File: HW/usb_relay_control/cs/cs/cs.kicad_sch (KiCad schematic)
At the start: 116 parts

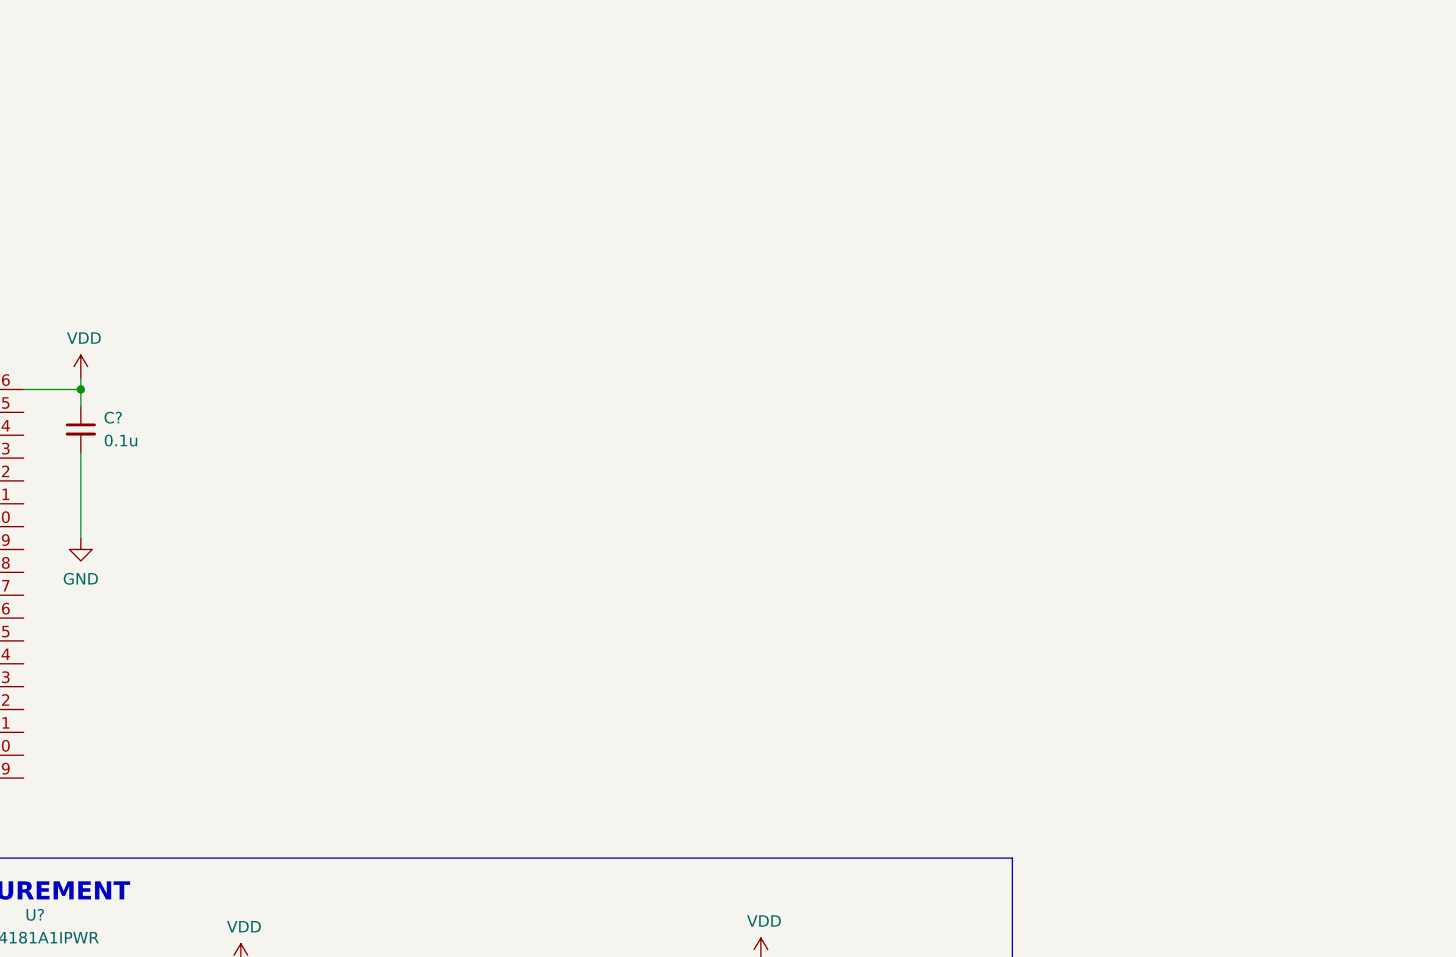
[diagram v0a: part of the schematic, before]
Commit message: ADD: AI antigravity review EMC according to IPC2221
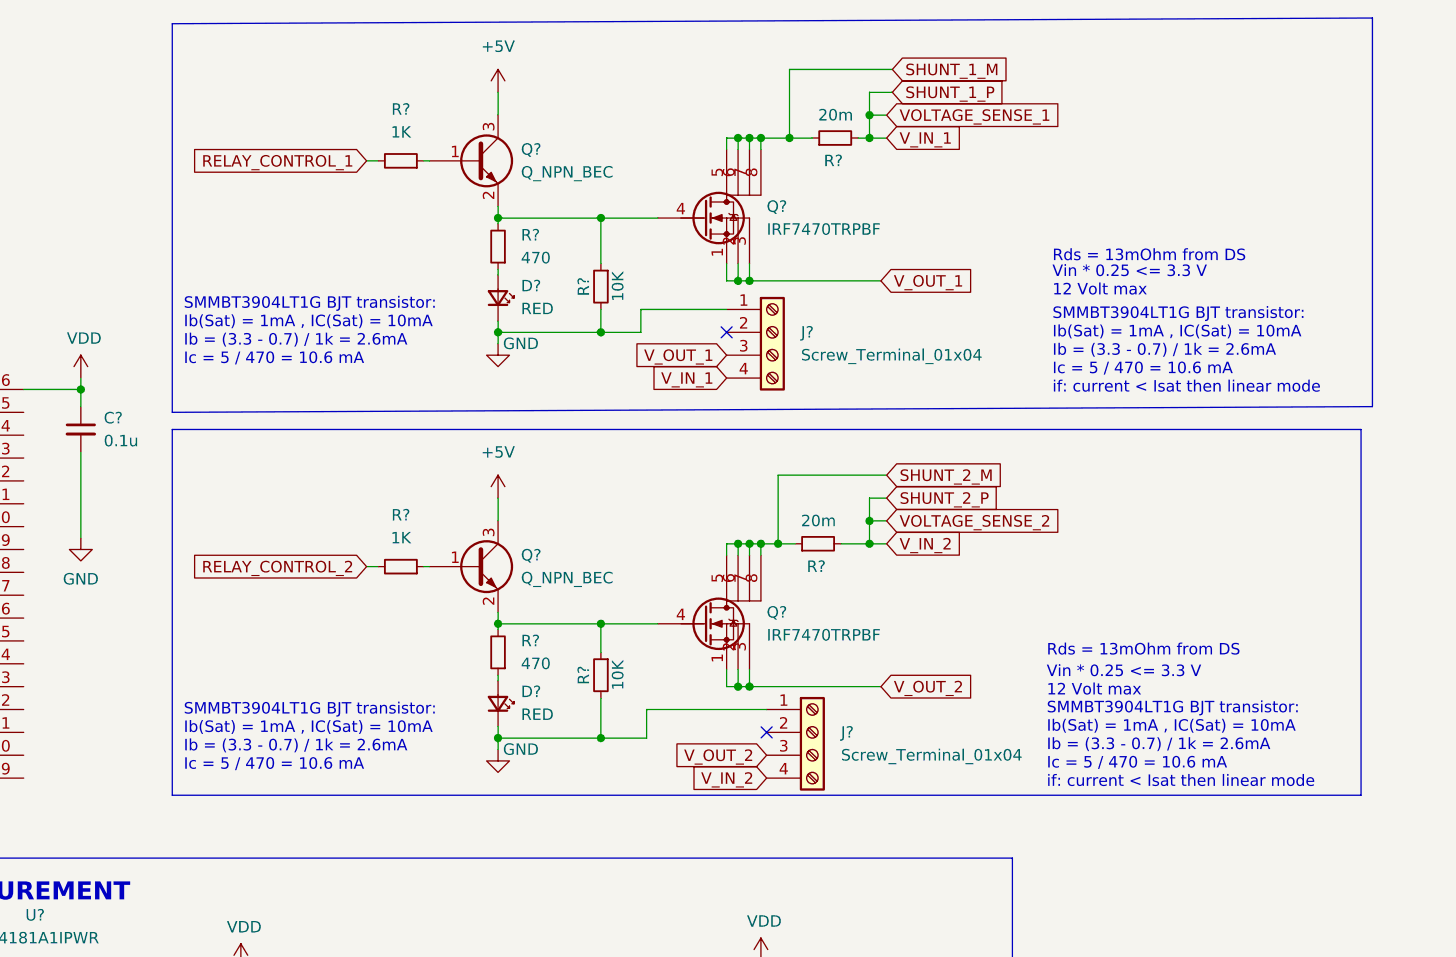
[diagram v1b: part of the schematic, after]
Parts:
- added D? (x2): RED, LED_SMD:LED_0805_2012Metric, symbol Device:LED_Small
- added J? (x2): Screw_Terminal_01x04, TerminalBlock_Phoenix:TerminalBlock_Phoenix_MKDS-1,5-4_1x04_P5.00mm_Horizontal, symbol Connector:Screw_Terminal_01x04
- added Q? (x2): Q_NPN_BEC, Package_TO_SOT_SMD:SOT-23, symbol Device:Q_NPN_BEC
- added Q? (x2): IRF7470TRPBF, IRF7470TRPBF:SOIC127P600X175-8N, symbol IRF7470TRPBF:IRF7470TRPBF
- added R? (x2): 1K, Resistor_SMD:R_0805_2012Metric, symbol Device:R_Small
- added R? (x2): 10K, Resistor_SMD:R_0805_2012Metric, symbol Device:R_Small
- added R? (x2): 470, Resistor_SMD:R_0805_2012Metric, symbol Device:R_Small
- added R? (x2): 20m, Resistor_SMD:R_1020_2550Metric, symbol Device:R_Small
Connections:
- net VOLTAGE_SENSE_1 is gone; now on net SHUNT_1_P: R?.1, R?.2, R?.2, R?.2, R?.2, R?.2
- net VOLTAGE_SENSE_2 is gone; now on net SHUNT_2_P: R?.2, R?.2, R?.2, R?.2
- net +5V: now also Q?.3 (C), Q?.3 (C)
- net GND: now also D?.1 (K), D?.1 (K), J?.1 (Pin_1), J?.1 (Pin_1), R?.2, R?.2
- net RELAY_CONTROL_1: now also R?.2
- net RELAY_CONTROL_2: now also R?.2
- net SHUNT_1_M: now also Q?.5 (D_1), Q?.6 (D_2), Q?.7 (D_3), Q?.8 (D_4), R?.1
- net SHUNT_1_P: now also J?.4 (Pin_4), R?.2
- net SHUNT_2_M: now also Q?.5 (D_1), Q?.6 (D_2), Q?.7 (D_3), Q?.8 (D_4), R?.1
- net SHUNT_2_P: now also J?.4 (Pin_4), R?.2
- new net: Q?.1 (B), R?.1 (x2)
- new net: Q?.2 (E), Q?.4 (G), R?.1, R?.2 (x2)
- new net: D?.2 (A), R?.1 (x2)
- new net V_OUT_1: J?.3 (Pin_3), Q?.1 (SN), Q?.2 (S_2), Q?.3 (S_3)
- new net V_OUT_2: J?.3 (Pin_3), Q?.1 (SN), Q?.2 (S_2), Q?.3 (S_3)
- no-connect marks 9 -> 11
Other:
- note added: "Rds = 13mOhm from DS"
- note added: "SMMBT3904LT1G BJT transistor: Ib(Sat) = 1mA , IC(Sat) = 10mA Ib = (3.3 - 0.7) / 1k = 2.6mA Ic = 5 / 470 = 10.6 mA"
- note added: "SMMBT3904LT1G BJT transistor: Ib(Sat) = 1mA , IC(Sat) = 10mA Ib = (3.3 - 0.7) / 1k = 2.6mA Ic = 5 / 470 = 10.6 mA if: current < Isat then linear mode"
